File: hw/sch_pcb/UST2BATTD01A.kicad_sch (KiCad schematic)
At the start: 8 parts, among them J1 SM03B-GHS-TB, J2 SM03B-GHS-TB

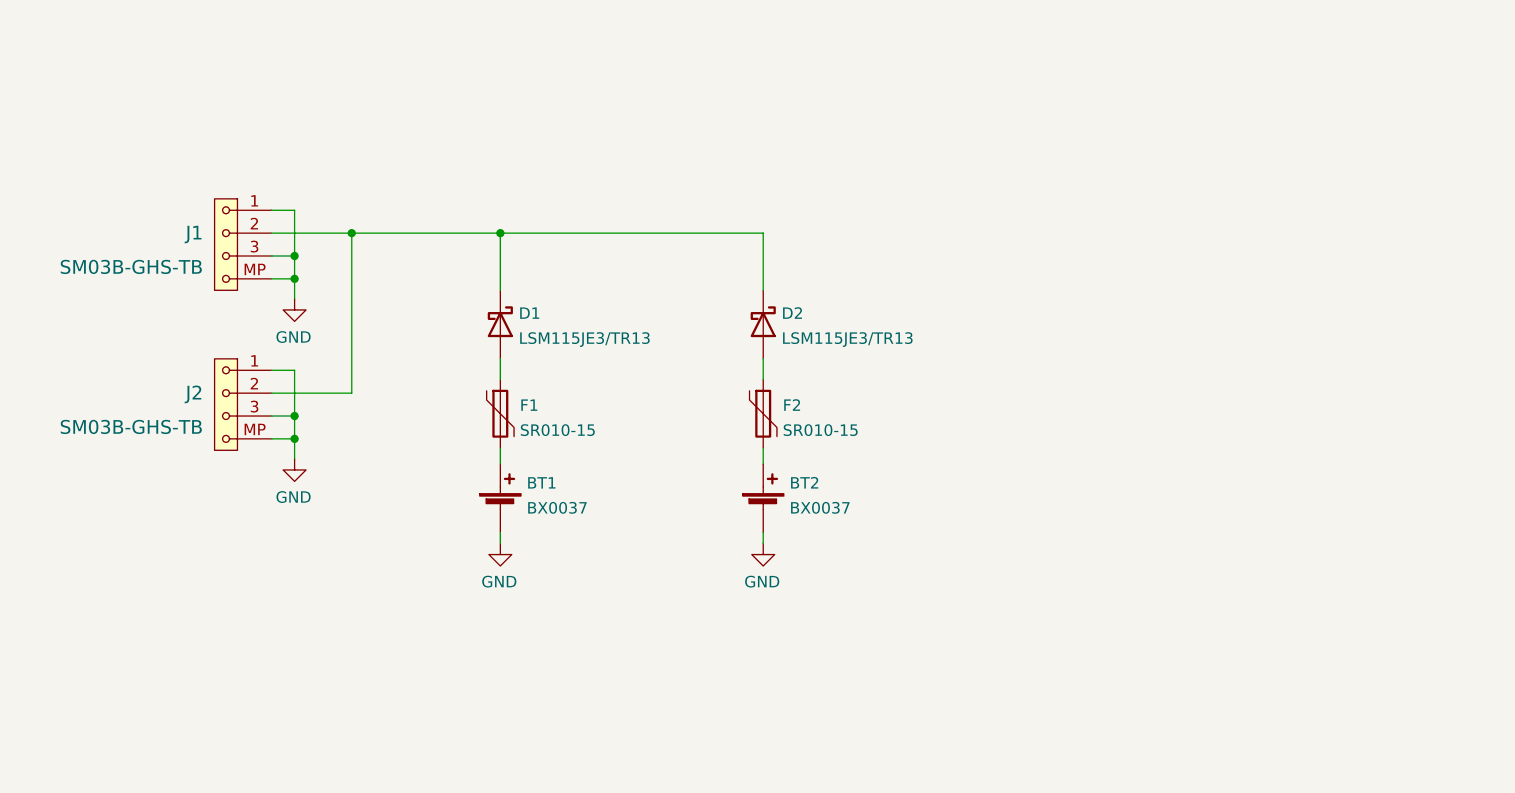
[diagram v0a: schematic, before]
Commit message: Edit PCB
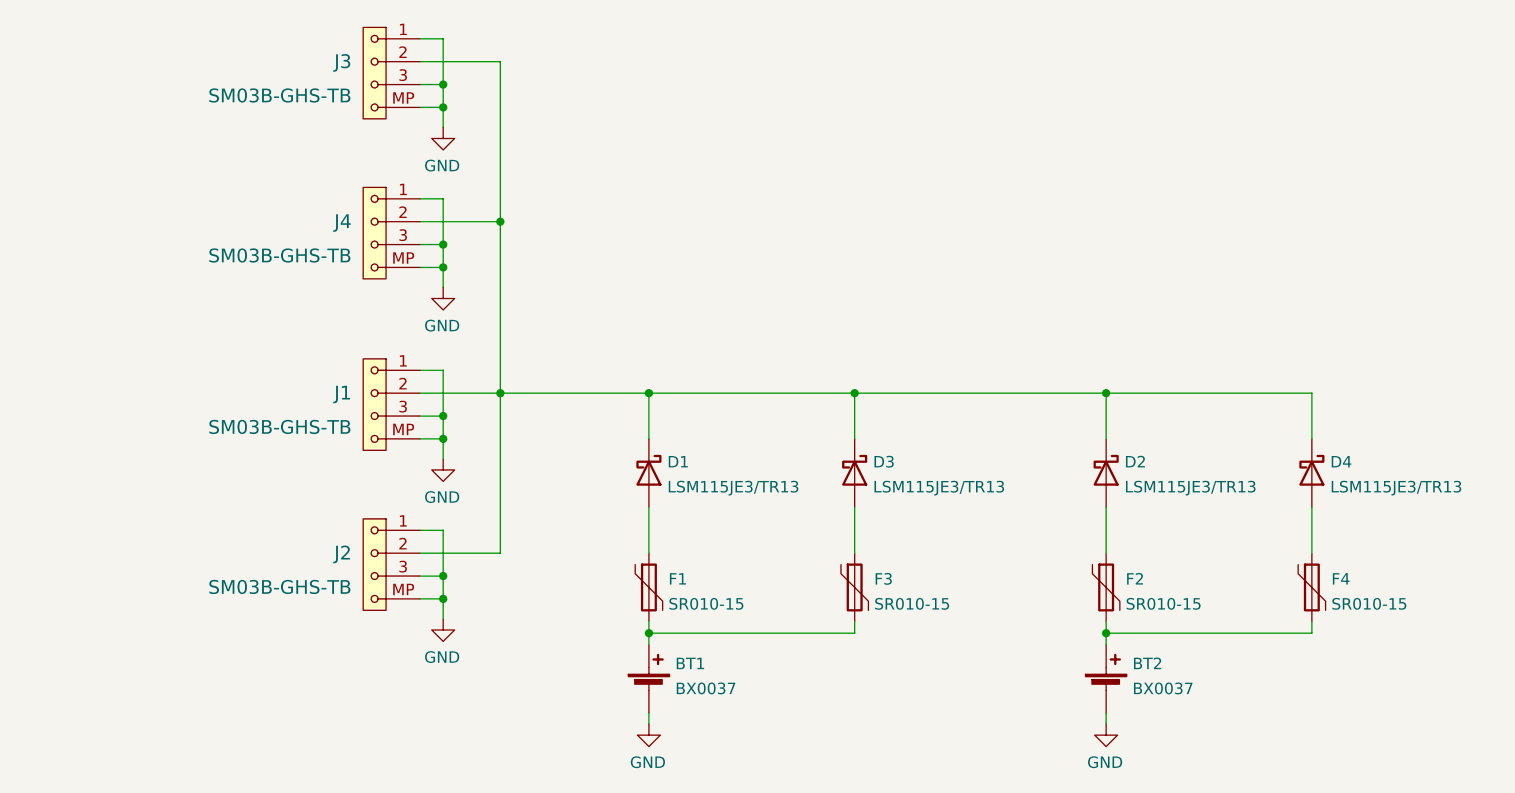
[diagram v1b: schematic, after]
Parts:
- added D3, D4: LSM115JE3/TR13, Diode_SMD:D_SMA_Handsoldering, symbol Device:D_Schottky
- added F3, F4: SR010-15, Fuse:Fuse_0805_2012Metric_Pad1.15x1.40mm_HandSolder, symbol Device:Polyfuse
- added J3, J4: SM03B-GHS-TB, Connector_JST:JST_GH_SM03B-GHS-TB_1x03-1MP_P1.25mm_Horizontal, symbol MLAB_CONNECTORS_JST:SM03B-GHS-TB
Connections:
- net GND: now also J3.1, J3.3, J3.MP, J4.1, J4.3, J4.MP
- net at D1.1 (K), D2.1 (K), J1.2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: now also D3.1 (K), D4.1 (K), J3.2, J4.2
- net at BT1.1 (+), F1.2: now also F3.2
- net at BT2.1 (+), F2.2: now also F4.2
- new net: D3.2 (A), F3.1
- new net: D4.2 (A), F4.1
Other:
- moved on the sheet: BT1, BT2, D1, D2, F1, F2, J1, J2
